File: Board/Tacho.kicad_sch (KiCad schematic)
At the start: 31 parts, among them Q3 WST2007, U1 KTH1601, U2 PY32F002AW15U

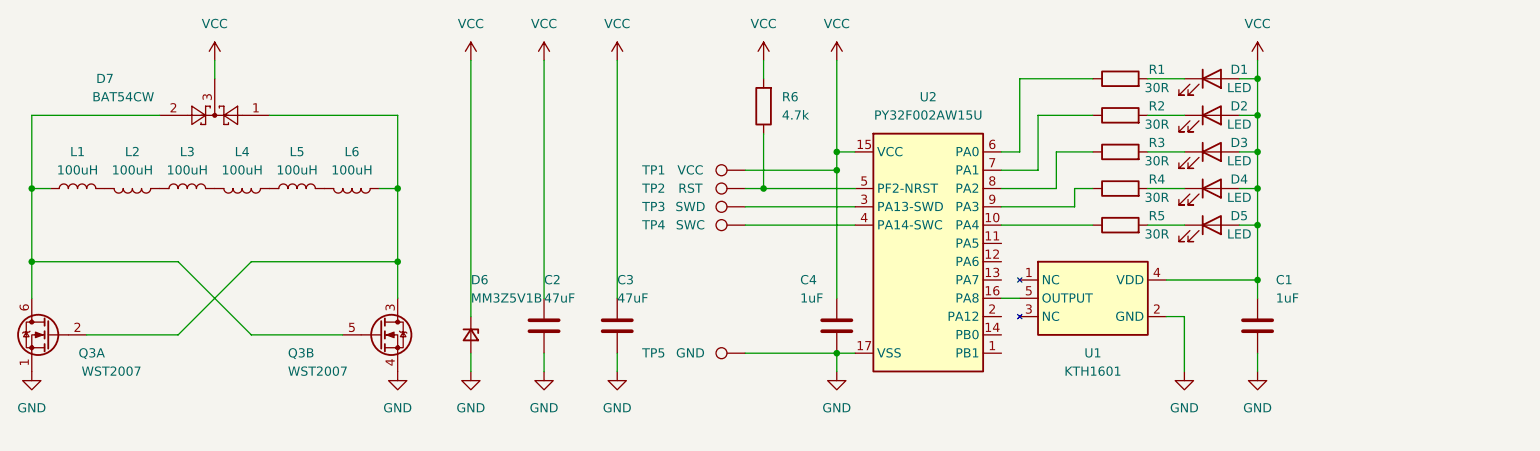
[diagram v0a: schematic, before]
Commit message: Layout finished
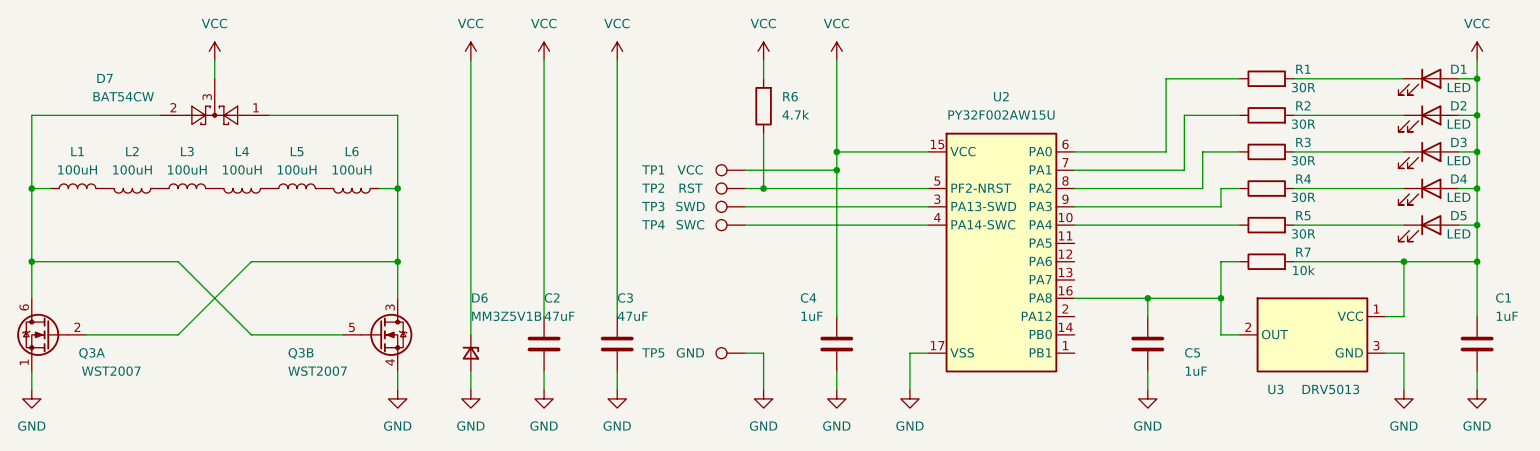
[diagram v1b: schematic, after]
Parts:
- removed U1: KTH1601, Package_TO_SOT_SMD:SOT-553, symbol USER:KTH1601
- added C5: 1uF, Capacitor_SMD:C_0402_1005Metric_Pad0.74x0.62mm_HandSolder, symbol Device:C
- added R7: 10k, Resistor_SMD:R_0402_1005Metric, symbol Device:R
- added U3: DRV5013, Package_TO_SOT_SMD:SOT-23, symbol USER:DRV5013
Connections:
- net GND: now also C5.2, U3.3 (GND)
- net VCC: now also R7.2, U3.1 (VCC)
- net at U2.16 (PA8): now also C5.1, R7.1, U3.2 (OUT)
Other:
- moved on the sheet: C1, C2, C3, C4, D1, D2, D3, D4, D5, D6, R1, R2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
